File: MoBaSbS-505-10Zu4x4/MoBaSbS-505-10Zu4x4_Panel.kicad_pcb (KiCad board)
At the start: 2 copper layers, 63.8 x 64.8 mm, 21 parts, among them J1 Conn_02x05_Odd_Even, J10 1, J11 2, J12 3, J13 4

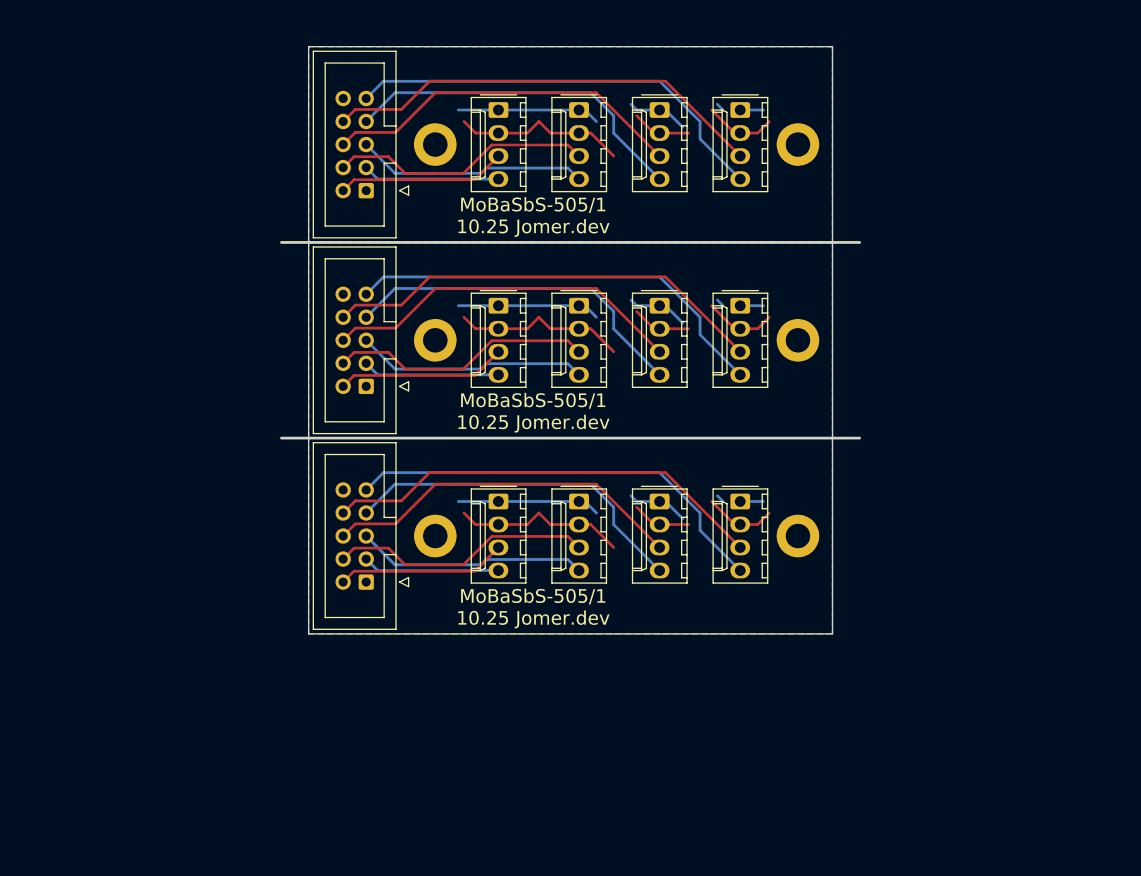
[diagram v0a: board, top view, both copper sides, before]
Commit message: Latest changes
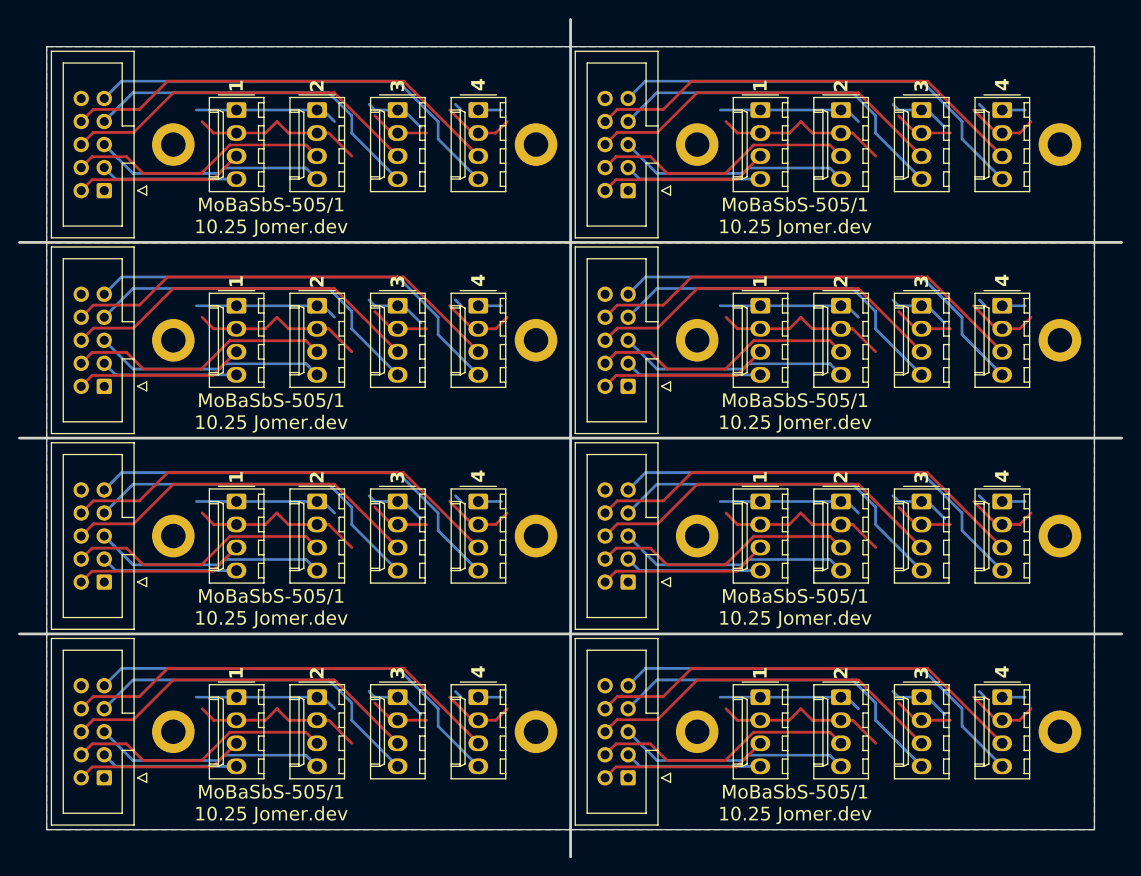
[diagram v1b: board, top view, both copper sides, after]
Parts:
- removed the H1 at (173.6, 74.0)
- removed the H1 at (173.6, 52.4)
- removed the H1 at (173.6, 30.8)
- removed the H3 at (133.6, 52.4)
- removed the H3 at (133.6, 74.0)
- removed the H3 at (133.6, 30.8)
- removed the J1 at (126.0, 35.9)
- removed the J1 at (126.0, 57.5)
- removed the J1 at (126.0, 79.1)
- removed the J10 at (140.5, 27.0)
- removed the J10 at (140.5, 48.6)
- removed the J10 at (140.5, 70.2)
- removed the J11 at (149.4, 48.6)
- removed the J11 at (149.4, 27.0)
- removed the J11 at (149.4, 70.2)
- removed the J12 at (158.3, 70.2)
- removed the J12 at (158.3, 27.0)
- removed the J12 at (158.3, 48.6)
- removed the J13 at (167.2, 48.6)
- removed the J13 at (167.2, 70.2)
- removed the J13 at (167.2, 27.0)
- added H1: MountingHole_Pad, MountingHole:MountingHole_2.7mm_M2.5_DIN965_Pad, F.Cu at (144.7, 95.6)
- added H1: MountingHole_Pad, MountingHole:MountingHole_2.7mm_M2.5_DIN965_Pad, F.Cu at (202.5, 74.0)
- added H1: MountingHole_Pad, MountingHole:MountingHole_2.7mm_M2.5_DIN965_Pad, F.Cu at (202.5, 52.4)
- added H1: MountingHole_Pad, MountingHole:MountingHole_2.7mm_M2.5_DIN965_Pad, F.Cu at (202.5, 30.8)
- added H1: MountingHole_Pad, MountingHole:MountingHole_2.7mm_M2.5_DIN965_Pad, F.Cu at (144.7, 30.8)
- added H1: MountingHole_Pad, MountingHole:MountingHole_2.7mm_M2.5_DIN965_Pad, F.Cu at (144.7, 74.0)
- added H1: MountingHole_Pad, MountingHole:MountingHole_2.7mm_M2.5_DIN965_Pad, F.Cu at (144.7, 52.4)
- added H1: MountingHole_Pad, MountingHole:MountingHole_2.7mm_M2.5_DIN965_Pad, F.Cu at (202.5, 95.6)
- added H3: MountingHole_Pad, MountingHole:MountingHole_2.7mm_M2.5_DIN965_Pad, F.Cu at (162.5, 30.8)
- added H3: MountingHole_Pad, MountingHole:MountingHole_2.7mm_M2.5_DIN965_Pad, F.Cu at (104.7, 95.6)
- added H3: MountingHole_Pad, MountingHole:MountingHole_2.7mm_M2.5_DIN965_Pad, F.Cu at (104.7, 30.8)
- added H3: MountingHole_Pad, MountingHole:MountingHole_2.7mm_M2.5_DIN965_Pad, F.Cu at (162.5, 52.4)
- added H3: MountingHole_Pad, MountingHole:MountingHole_2.7mm_M2.5_DIN965_Pad, F.Cu at (162.5, 95.6)
- added H3: MountingHole_Pad, MountingHole:MountingHole_2.7mm_M2.5_DIN965_Pad, F.Cu at (104.7, 74.0)
- added H3: MountingHole_Pad, MountingHole:MountingHole_2.7mm_M2.5_DIN965_Pad, F.Cu at (162.5, 74.0)
- added H3: MountingHole_Pad, MountingHole:MountingHole_2.7mm_M2.5_DIN965_Pad, F.Cu at (104.7, 52.4)
- added J1: Conn_02x05_Odd_Even, Connector_IDC:IDC-Header_2x05_P2.54mm_Vertical, F.Cu at (97.1, 35.9)
- added J1: Conn_02x05_Odd_Even, Connector_IDC:IDC-Header_2x05_P2.54mm_Vertical, F.Cu at (154.8, 100.6)
- added J1: Conn_02x05_Odd_Even, Connector_IDC:IDC-Header_2x05_P2.54mm_Vertical, F.Cu at (97.1, 79.1)
- added J1: Conn_02x05_Odd_Even, Connector_IDC:IDC-Header_2x05_P2.54mm_Vertical, F.Cu at (154.8, 35.9)
- added J1: Conn_02x05_Odd_Even, Connector_IDC:IDC-Header_2x05_P2.54mm_Vertical, F.Cu at (154.8, 79.1)
- added J1: Conn_02x05_Odd_Even, Connector_IDC:IDC-Header_2x05_P2.54mm_Vertical, F.Cu at (97.1, 57.5)
- added J1: Conn_02x05_Odd_Even, Connector_IDC:IDC-Header_2x05_P2.54mm_Vertical, F.Cu at (154.8, 57.5)
- added J1: Conn_02x05_Odd_Even, Connector_IDC:IDC-Header_2x05_P2.54mm_Vertical, F.Cu at (97.1, 100.6)
- added J10: 1, Connector_Molex:Molex_KK-254_AE-6410-04A_1x04_P2.54mm_Vertical, F.Cu at (111.7, 91.8)
- added J10: 1, Connector_Molex:Molex_KK-254_AE-6410-04A_1x04_P2.54mm_Vertical, F.Cu at (111.7, 27.0)
- added J10: 1, Connector_Molex:Molex_KK-254_AE-6410-04A_1x04_P2.54mm_Vertical, F.Cu at (169.4, 91.8)
- added J10: 1, Connector_Molex:Molex_KK-254_AE-6410-04A_1x04_P2.54mm_Vertical, F.Cu at (169.4, 27.0)
- added J10: 1, Connector_Molex:Molex_KK-254_AE-6410-04A_1x04_P2.54mm_Vertical, F.Cu at (169.4, 70.2)
- added J10: 1, Connector_Molex:Molex_KK-254_AE-6410-04A_1x04_P2.54mm_Vertical, F.Cu at (111.7, 48.6)
- added J10: 1, Connector_Molex:Molex_KK-254_AE-6410-04A_1x04_P2.54mm_Vertical, F.Cu at (169.4, 48.6)
- added J10: 1, Connector_Molex:Molex_KK-254_AE-6410-04A_1x04_P2.54mm_Vertical, F.Cu at (111.7, 70.2)
- added J11: 2, Connector_Molex:Molex_KK-254_AE-6410-04A_1x04_P2.54mm_Vertical, F.Cu at (178.3, 48.6)
- added J11: 2, Connector_Molex:Molex_KK-254_AE-6410-04A_1x04_P2.54mm_Vertical, F.Cu at (178.3, 27.0)
- added J11: 2, Connector_Molex:Molex_KK-254_AE-6410-04A_1x04_P2.54mm_Vertical, F.Cu at (178.3, 70.2)
- added J11: 2, Connector_Molex:Molex_KK-254_AE-6410-04A_1x04_P2.54mm_Vertical, F.Cu at (120.5, 48.6)
- added J11: 2, Connector_Molex:Molex_KK-254_AE-6410-04A_1x04_P2.54mm_Vertical, F.Cu at (120.5, 91.8)
- added J11: 2, Connector_Molex:Molex_KK-254_AE-6410-04A_1x04_P2.54mm_Vertical, F.Cu at (120.5, 27.0)
- added J11: 2, Connector_Molex:Molex_KK-254_AE-6410-04A_1x04_P2.54mm_Vertical, F.Cu at (120.5, 70.2)
- added J11: 2, Connector_Molex:Molex_KK-254_AE-6410-04A_1x04_P2.54mm_Vertical, F.Cu at (178.3, 91.8)
- added J12: 3, Connector_Molex:Molex_KK-254_AE-6410-04A_1x04_P2.54mm_Vertical, F.Cu at (129.4, 27.0)
- added J12: 3, Connector_Molex:Molex_KK-254_AE-6410-04A_1x04_P2.54mm_Vertical, F.Cu at (129.4, 91.8)
- added J12: 3, Connector_Molex:Molex_KK-254_AE-6410-04A_1x04_P2.54mm_Vertical, F.Cu at (187.2, 48.6)
- added J12: 3, Connector_Molex:Molex_KK-254_AE-6410-04A_1x04_P2.54mm_Vertical, F.Cu at (129.4, 70.2)
- added J12: 3, Connector_Molex:Molex_KK-254_AE-6410-04A_1x04_P2.54mm_Vertical, F.Cu at (187.2, 70.2)
- added J12: 3, Connector_Molex:Molex_KK-254_AE-6410-04A_1x04_P2.54mm_Vertical, F.Cu at (129.4, 48.6)
- added J12: 3, Connector_Molex:Molex_KK-254_AE-6410-04A_1x04_P2.54mm_Vertical, F.Cu at (187.2, 91.8)
- added J12: 3, Connector_Molex:Molex_KK-254_AE-6410-04A_1x04_P2.54mm_Vertical, F.Cu at (187.2, 27.0)
- added J13: 4, Connector_Molex:Molex_KK-254_AE-6410-04A_1x04_P2.54mm_Vertical, F.Cu at (138.3, 91.8)
- added J13: 4, Connector_Molex:Molex_KK-254_AE-6410-04A_1x04_P2.54mm_Vertical, F.Cu at (196.1, 48.6)
- added J13: 4, Connector_Molex:Molex_KK-254_AE-6410-04A_1x04_P2.54mm_Vertical, F.Cu at (138.3, 48.6)
- added J13: 4, Connector_Molex:Molex_KK-254_AE-6410-04A_1x04_P2.54mm_Vertical, F.Cu at (196.1, 70.2)
- added J13: 4, Connector_Molex:Molex_KK-254_AE-6410-04A_1x04_P2.54mm_Vertical, F.Cu at (196.1, 27.0)
- added J13: 4, Connector_Molex:Molex_KK-254_AE-6410-04A_1x04_P2.54mm_Vertical, F.Cu at (196.1, 91.8)
- added J13: 4, Connector_Molex:Molex_KK-254_AE-6410-04A_1x04_P2.54mm_Vertical, F.Cu at (138.3, 70.2)
- added J13: 4, Connector_Molex:Molex_KK-254_AE-6410-04A_1x04_P2.54mm_Vertical, F.Cu at (138.3, 27.0)
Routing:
- net Board_5-/PIN_7: track 0.00 -> 49.1 mm
- net Board_4-/PIN_7: track 0.00 -> 49.1 mm
- net Board_7-/PIN_7: track 0.00 -> 49.1 mm
- net Board_6-/PIN_7: track 0.00 -> 49.1 mm
- net Board_3-/PIN_7: track 0.00 -> 49.1 mm
- net Board_7-/PIN_8: track 0.00 -> 47.6 mm
- net Board_3-/PIN_8: track 0.00 -> 47.6 mm
- net Board_5-/PIN_8: track 0.00 -> 47.6 mm
- net Board_6-/PIN_8: track 0.00 -> 47.6 mm
- net Board_4-/PIN_8: track 0.00 -> 47.6 mm
- net Board_7-/PIN_5: track 0.00 -> 40.2 mm
- net Board_6-/PIN_5: track 0.00 -> 40.2 mm
- net Board_3-/PIN_5: track 0.00 -> 40.2 mm
- net Board_5-/PIN_5: track 0.00 -> 40.2 mm
- net Board_4-/PIN_5: track 0.00 -> 40.2 mm
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- added copper zone on F.Cu, net Board_3-/GND
- added copper zone on B.Cu, net Board_3-/POWER
- added copper zone on F.Cu, net Board_4-/GND
- added copper zone on B.Cu, net Board_4-/POWER
- added copper zone on F.Cu, net Board_5-/GND
- added copper zone on B.Cu, net Board_5-/POWER
- added copper zone on F.Cu, net Board_6-/GND
- added copper zone on B.Cu, net Board_6-/POWER
- added copper zone on F.Cu, net Board_7-/GND
- added copper zone on B.Cu, net Board_7-/POWER
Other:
- board size 63.8 x 64.8 mm -> 121.6 x 92.4 mm
- board text added: "1"
- board text added: "2"
- board text added: "3"
- board text added: "4"
